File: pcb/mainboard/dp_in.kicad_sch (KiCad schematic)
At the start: 33 parts, among them J1 XUNPU TYPEC-324G-ACP24, U16 USBLC6-2P6, U17 FUSB302BMPX, U18 CBTL02043A, U19 PTN3460

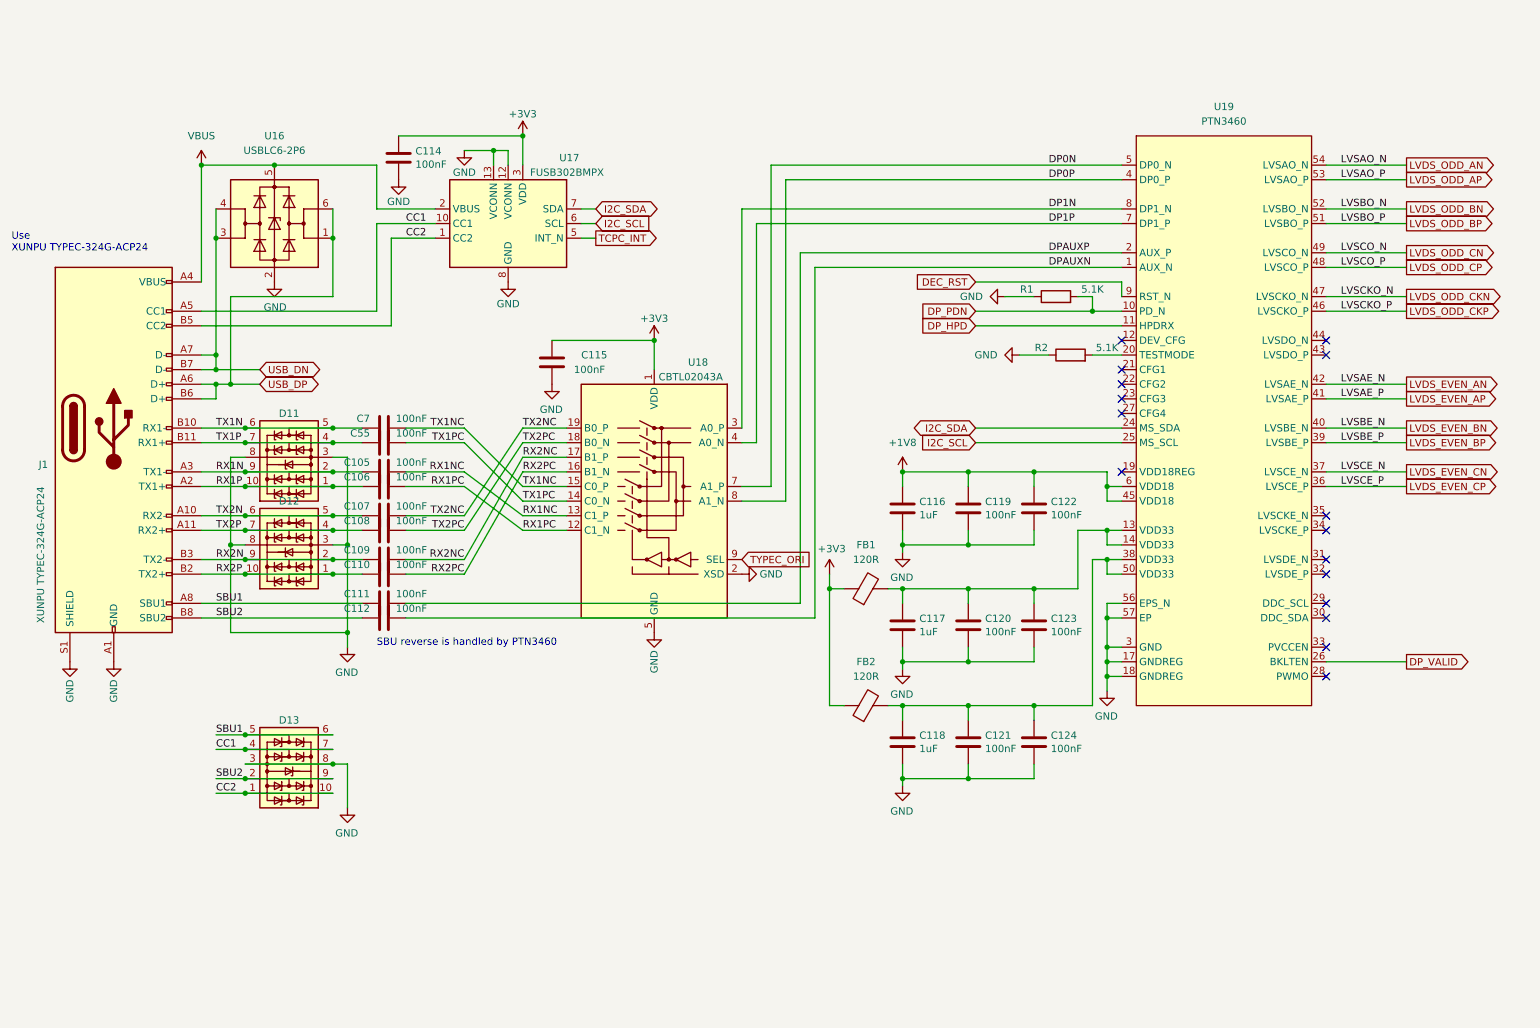
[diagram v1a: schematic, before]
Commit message: PCB r0p9
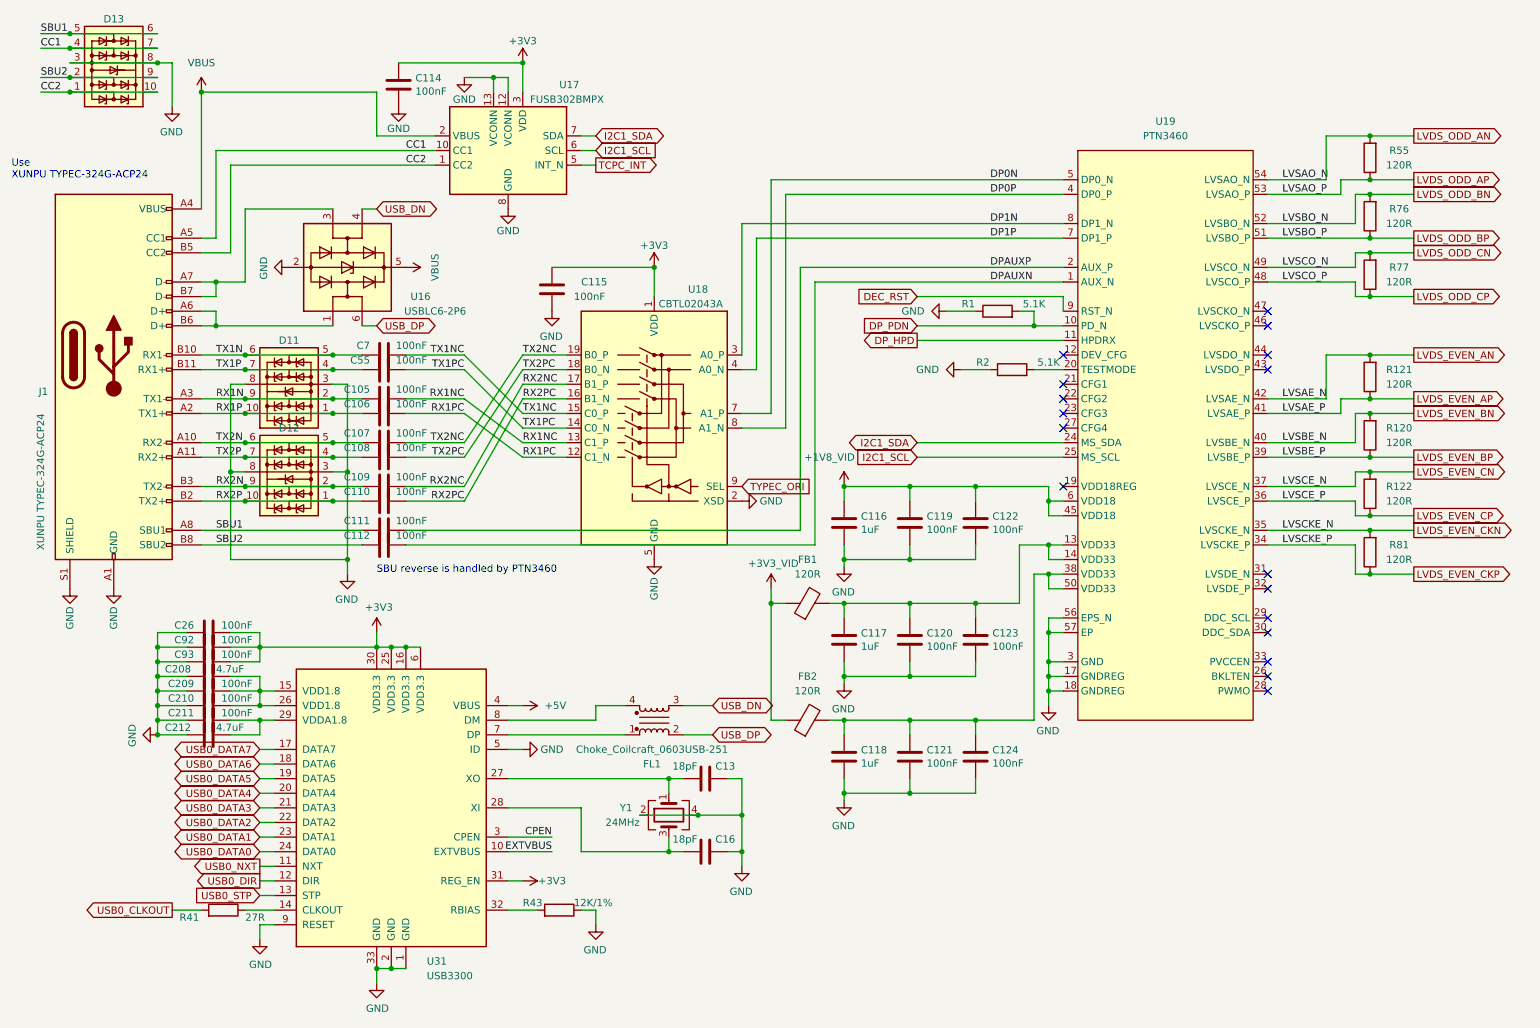
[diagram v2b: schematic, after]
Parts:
- added C13, C16: 18pF, Capacitor_SMD:C_0402_1005Metric, symbol Device:C
- added C208, C212: 4.7uF, Capacitor_SMD:C_0603_1608Metric, symbol Device:C
- added C209, C210, C211, C26, C92, C93: 100nF, Capacitor_SMD:C_0402_1005Metric, symbol Device:C
- added FL1: Choke_Coilcraft_0603USB-251, Inductor_SMD:L_CommonModeChoke_Coilcraft_0603USB, symbol Filter:Choke_Coilcraft_0603USB-251
- added R120, R121, R122, R55, R76, R77, R81: 120R, Resistor_SMD:R_0402_1005Metric, symbol Device:R
- added R41: 27R, Resistor_SMD:R_0402_1005Metric, symbol Device:R
- added R43: 12K/1%, Resistor_SMD:R_0402_1005Metric, symbol Device:R
- added U31: USB3300, Package_DFN_QFN:QFN-32-1EP_5x5mm_P0.5mm_EP3.3x3.3mm, symbol Interface_USB:USB3300-EZK
- added Y1: 24MHz, Crystal:Crystal_SMD_3225-4Pin_3.2x2.5mm, symbol Device:Crystal_GND24
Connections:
- net +3V3: now also C26.2, C92.2, C93.2, U31.16 (VDD3.3), U31.25 (VDD3.3), U31.30 (VDD3.3), U31.31 (REG_EN), U31.6 (VDD3.3); no longer FB1.1, FB2.1
- net GND: now also C13.2, C16.2, C208.2, C209.1, C210.1, C211.1, C212.2, C26.1, C92.1, C93.1, R43.1, U31.1 (GND), U31.2 (GND), U31.33 (GND), U31.5 (ID), U31.9 (RESET), Y1.2, Y1.4
- net LVDS_EVEN_AN: now also R121.2
- net LVDS_EVEN_AP: now also R121.1
- net LVDS_EVEN_BN: now also R120.2
- net LVDS_EVEN_BP: now also R120.1
- net LVDS_EVEN_CN: now also R122.2
- net LVDS_EVEN_CP: now also R122.1
- net LVDS_ODD_AN: now also R55.2
- net LVDS_ODD_AP: now also R55.1
- net LVDS_ODD_BN: now also R76.2
- net LVDS_ODD_BP: now also R76.1
- net LVDS_ODD_CN: now also R77.2
- net LVDS_ODD_CP: now also R77.1
- net USB_DN: now also FL1.3; no longer J1.A7 (D-), J1.B7 (D-), U16.3 (I/O2)
- net USB_DP: now also FL1.2; no longer J1.A6 (D+), J1.B6 (D+), U16.1 (I/O1)
- net LVDS_EVEN_CKP: now reaches U19.34 (LVSCKE_P)
- net LVDS_EVEN_CKP: now also R81.1
- net LVDS_EVEN_CKN: now reaches U19.35 (LVSCKE_N)
- net LVDS_EVEN_CKN: now also R81.2
- net +1V8 renamed +1V8_VID
- net DP_VALID: no longer names the net of U19.26 (BKLTEN)
- net I2C_SCL renamed I2C1_SCL
- net I2C_SDA renamed I2C1_SDA
- net LVDS_ODD_CKN: no longer names the net of U19.47 (LVSCKO_N)
- net LVDS_ODD_CKP: no longer names the net of U19.46 (LVSCKO_P)
- new net: C211.2, C212.1, U31.29 (VDDA1.8)
- new net: R41.1, U31.14 (CLKOUT)
- new net: C208.1, C209.2, C210.2, U31.15 (VDD1.8), U31.26 (VDD1.8)
- new net: C13.1, U31.27 (XO), Y1.1
- new net: C16.1, U31.28 (XI), Y1.3
- new net: R43.2, U31.32 (RBIAS)
- new net: FL1.1, U31.7 (DP)
- new net: FL1.4, U31.8 (DM)
- new net: J1.A6 (D+), J1.B6 (D+), U16.1 (I/O1)
- new net: J1.A7 (D-), J1.B7 (D-), U16.3 (I/O2)
- new net +3V3_VID: FB1.1, FB2.1
- new net +5V: U31.4 (VBUS)
- new net CPEN: U31.3 (CPEN)
- new net EXTVBUS: U31.10 (EXTVBUS)
- new net USB0_CLKOUT: R41.2
- new net USB0_DATA0: U31.24 (DATA0)
- new net USB0_DATA1: U31.23 (DATA1)
- new net USB0_DATA2: U31.22 (DATA2)
- new net USB0_DATA3: U31.21 (DATA3)
- new net USB0_DATA4: U31.20 (DATA4)
- new net USB0_DATA5: U31.19 (DATA5)
- new net USB0_DATA6: U31.18 (DATA6)
- new net USB0_DATA7: U31.17 (DATA7)
- new net USB0_DIR: U31.12 (DIR)
- new net USB0_NXT: U31.11 (NXT)
- new net USB0_STP: U31.13 (STP)
- no-connect marks 16 -> 17
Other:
- moved on the sheet: C105, C106, C107, C108, C109, C110, C111, C112, C114, C115, C116, C117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

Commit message: PCB r0p10 wip
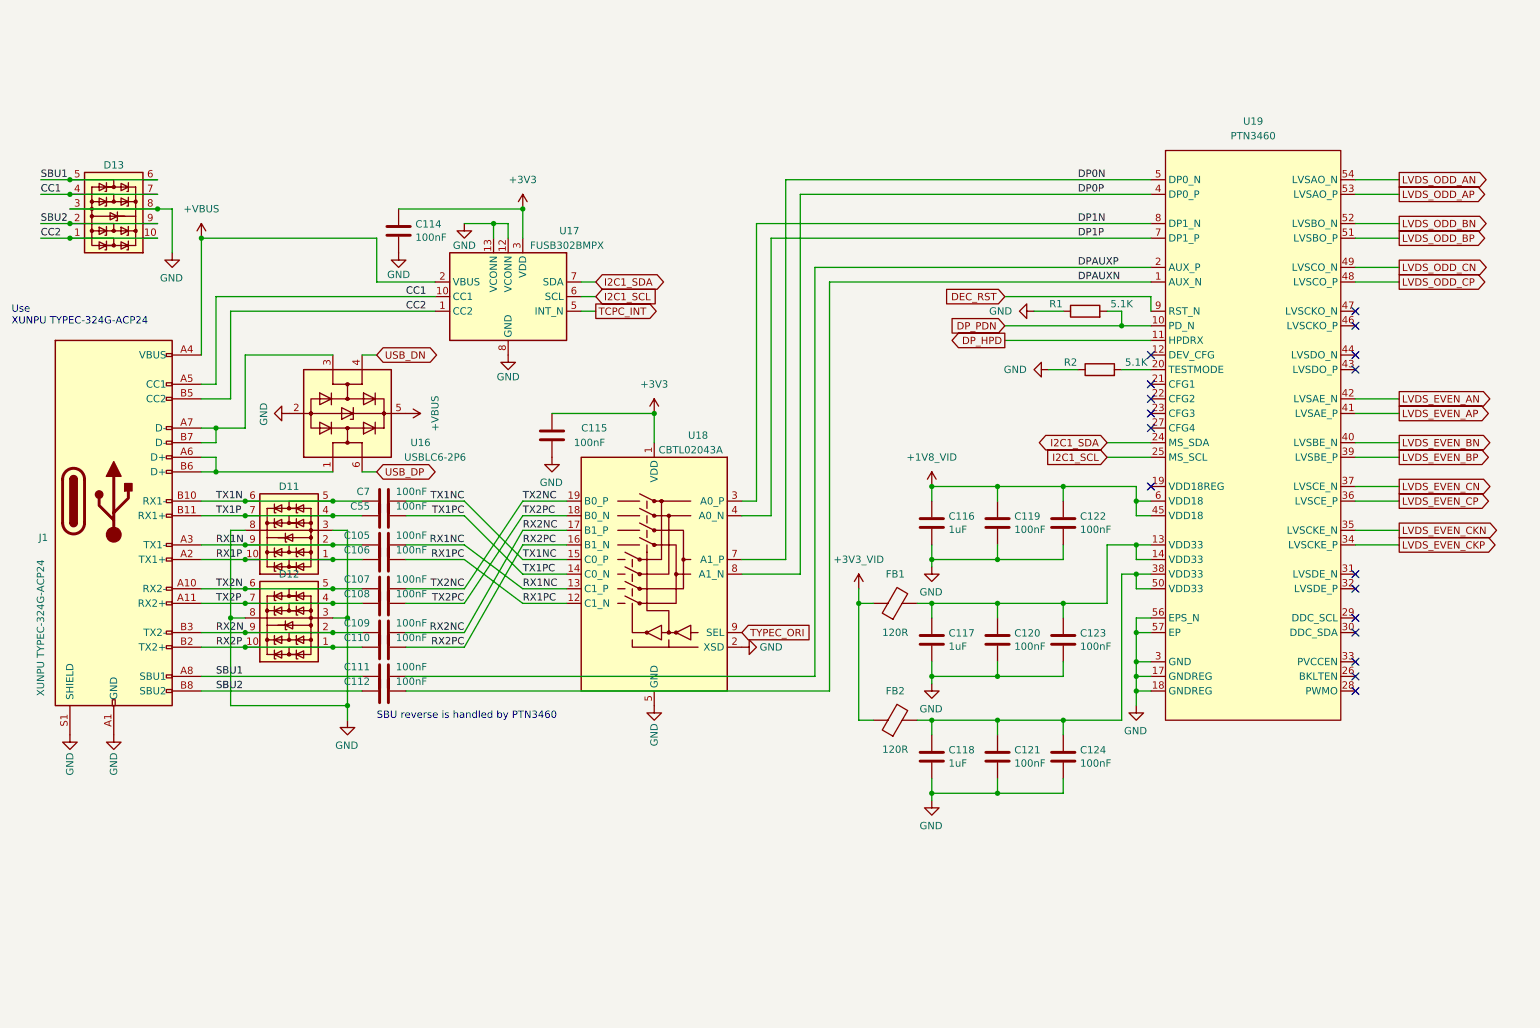
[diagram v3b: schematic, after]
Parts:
- removed C13, C16: 18pF, Capacitor_SMD:C_0402_1005Metric, symbol Device:C
- removed C208, C212: 4.7uF, Capacitor_SMD:C_0603_1608Metric, symbol Device:C
- removed C209, C210, C211, C26, C92, C93: 100nF, Capacitor_SMD:C_0402_1005Metric, symbol Device:C
- removed FL1: Choke_Coilcraft_0603USB-251, Inductor_SMD:L_CommonModeChoke_Coilcraft_0603USB, symbol Filter:Choke_Coilcraft_0603USB-251
- removed R120, R121, R122, R55, R76, R77, R81: 120R, Resistor_SMD:R_0402_1005Metric, symbol Device:R
- removed R41: 27R, Resistor_SMD:R_0402_1005Metric, symbol Device:R
- removed R43: 12K/1%, Resistor_SMD:R_0402_1005Metric, symbol Device:R
- removed U31: USB3300, Package_DFN_QFN:QFN-32-1EP_5x5mm_P0.5mm_EP3.3x3.3mm, symbol Interface_USB:USB3300-EZK
- removed Y1: 24MHz, Crystal:Crystal_SMD_3225-4Pin_3.2x2.5mm, symbol Device:Crystal_GND24
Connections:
- net VBUS renamed +VBUS
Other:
- moved on the sheet: C105, C106, C107, C108, C109, C110, C111, C112, C114, C115, C116, C117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
